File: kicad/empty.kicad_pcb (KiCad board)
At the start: 2 copper layers, 160 x 100.3 mm, 5 parts, among them P5 CONN_02X25

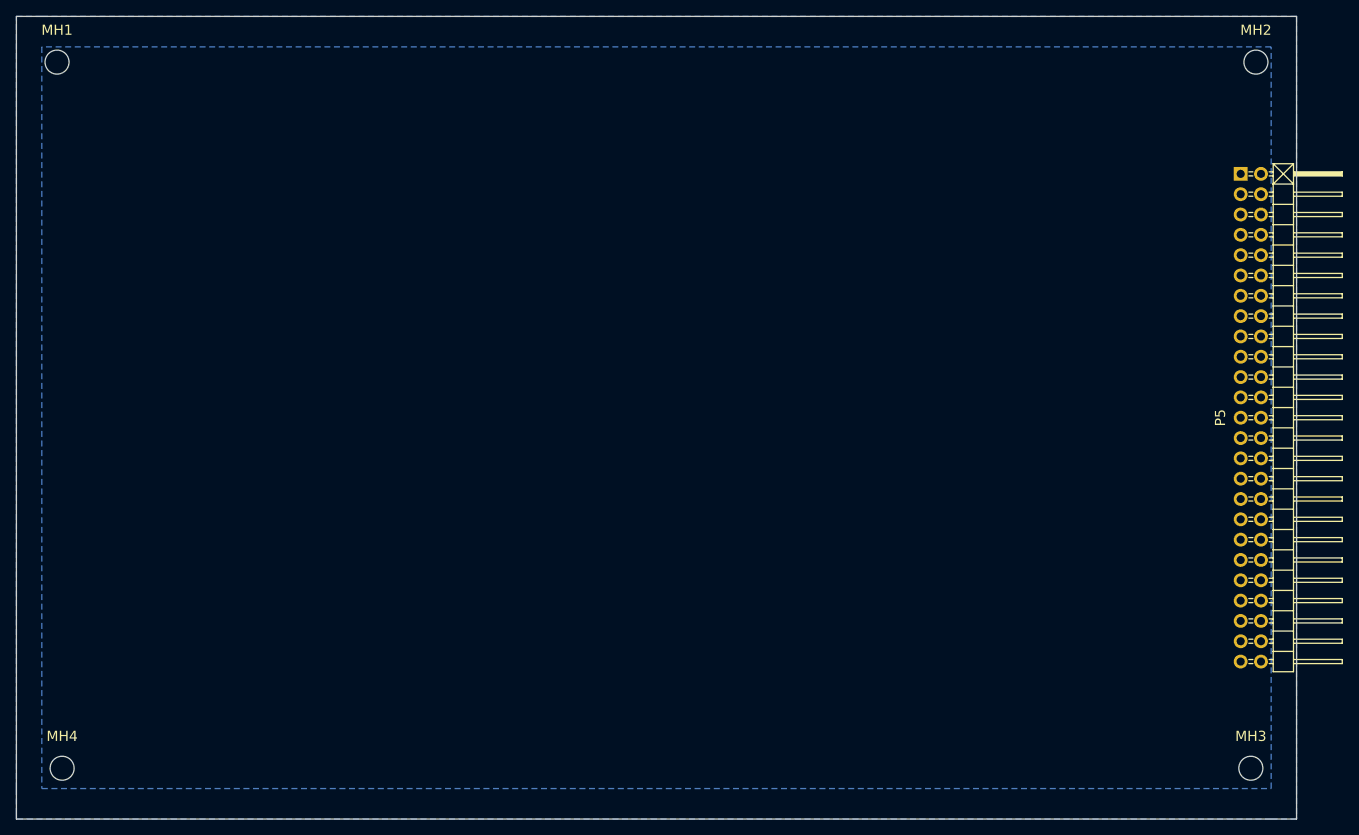
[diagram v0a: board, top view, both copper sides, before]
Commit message: update
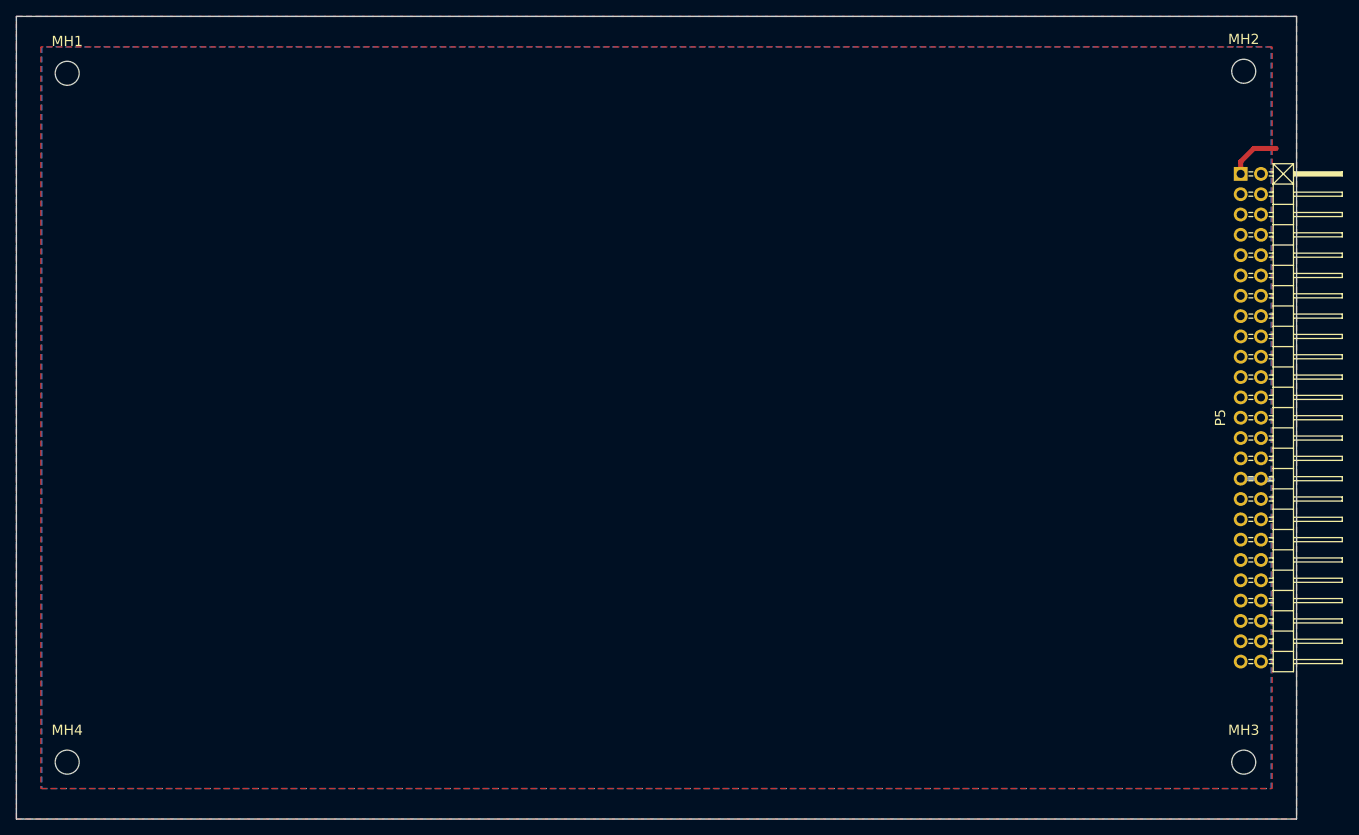
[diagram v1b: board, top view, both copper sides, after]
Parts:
- moved MH2 1.91 mm to (215.6, 52.6)
- moved MH1 1.89 mm to (68.6, 52.8)
- moved MH3 1.17 mm to (215.6, 138.9)
- moved MH4 0.99 mm to (68.6, 138.9)
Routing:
- net VCC: track 0.00 -> 6.65 mm
- net GND: track 0.00 -> 3.99 mm
- added copper zone on F.Cu, net VCC
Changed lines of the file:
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@@
   (general
     (links 1)
-    (no_connects 1)
-    (area 6.781073 60.8965 204.770447 161.41446)
+    (no_connects 0)
+    (area 44.246073 45.6565 242.235447 146.17446)
     (thickness 1.6)
     (drawings 4)
-    (tracks 0)
+    (tracks 6)
     (zones 0)
     (modules 5)
@@
     (add_net VCC)
   )
-  (module Pin_Headers:Pin_Header_Angled_2x25 (layer F.Cu)
+  (module Pin_Headers:Pin_Header_Angled_2x25 locked (layer F.Cu)
     (at 216.535 95.885 270)
     (descr "Through hole pin header")
@@
     )
   )
-  (module Mounting_Holes:MountingHole_3mm (layer F.Cu)
-    (at 67.31 51.435)
+  (module Mounting_Holes:MountingHole_3mm locked (layer F.Cu)
+    (at 68.58 52.832)
     (descr "Mounting hole, Befestigungsbohrung, 3mm, No Annular, Kein Restring,")
     (tags "Mounting hole, Befestigungsbohrung, 3mm, No Annular, Kein Restring,")
@@
     (pad 1 thru_hole circle (at 0 0) (size 2.99974 2.99974) (drill 2.99974) (layers))
   )
-  (module Mounting_Holes:MountingHole_3mm (layer F.Cu)
-    (at 217.17 51.435)
+  (module Mounting_Holes:MountingHole_3mm locked (layer F.Cu)
+    (at 215.646 52.578)
     (descr "Mounting hole, Befestigungsbohrung, 3mm, No Annular, Kein Restring,")
     (tags "Mounting hole, Befestigungsbohrung, 3mm, No Annular, Kein Restring,")
@@
     (pad 1 thru_hole circle (at 0 0) (size 2.99974 2.99974) (drill 2.99974) (layers))
   )
-  (module Mounting_Holes:MountingHole_3mm (layer F.Cu)
-    (at 67.945 139.7)
+  (module Mounting_Holes:MountingHole_3mm locked (layer F.Cu)
+    (at 68.58 138.938)
     (descr "Mounting hole, Befestigungsbohrung, 3mm, No Annular, Kein Restring,")
     (tags "Mounting hole, Befestigungsbohrung, 3mm, No Annular, Kein Restring,")
@@
     (pad 1 thru_hole circle (at 0 0) (size 2.99974 2.99974) (drill 2.99974) (layers))
   )
-  (module Mounting_Holes:MountingHole_3mm (layer F.Cu)
-    (at 216.535 139.7)
+  (module Mounting_Holes:MountingHole_3mm locked (layer F.Cu)
+    (at 215.646 138.938)
     (descr "Mounting hole, Befestigungsbohrung, 3mm, No Annular, Kein Restring,")
     (tags "Mounting hole, Befestigungsbohrung, 3mm, No Annular, Kein Restring,")
@@
   (gr_line (start 222.25 45.72) (end 222.25 146.05) (angle 90) (layer Edge.Cuts) (width 0.1))
   (gr_line (start 62.23 45.72) (end 222.25 45.72) (angle 90) (layer Edge.Cuts) (width 0.1))
+  (segment (start 215.265 103.505) (end 217.805 103.505) (width 0.635) (layer B.Cu) (net 1) (status C00000))
+  (segment (start 217.805 103.505) (end 217.932 103.632) (width 0.635) (layer B.Cu) (net 1) (status C00000))
+  (segment (start 217.932 103.632) (end 219.202 103.632) (width 0.635) (layer B.Cu) (net 1) (status 400000))
+  (segment (start 215.265 65.405) (end 215.265 63.881) (width 0.635) (layer F.Cu) (net 2) (status 400000))
+  (segment (start 216.916 62.23) (end 219.71 62.23) (width 0.635) (layer F.Cu) (net 2))
+  (segment (start 215.265 63.881) (end 216.916 62.23) (width 0.635) (layer F.Cu) (net 2))
   (zone (net 1) (net_name GND) (layer B.Cu) (hatch edge 0.508)
     (connect_pads (clearance 0.508))
@@
       )
     )
+  )
+  (zone (net 2) (net_name VCC) (layer F.Cu) (hatch edge 0.508)
+    (connect_pads (clearance 0.508))
+    (min_thickness 0.254)
+    (fill (arc_segments 16) (thermal_gap 0.508) (thermal_bridge_width 0.508))
+    (polygon
+      (pts
+        (xy 222.25 146.05) (xy 65.278 146.05) (xy 62.23 146.05) (xy 62.23 49.53) (xy 62.23 45.72)
+        (xy 222.25 45.72) (xy 222.25 49.53) (xy 222.25 142.24) (xy 222.25 142.494) (xy 222.25 146.05)
+      )
+    )
+    (polygon
+      (pts        (xy 219.202 142.24) (xy 219.202 49.53) (xy 65.278 49.53) (xy 65.278 142.24) (xy 219.202 142.24)
+      )
+    )
